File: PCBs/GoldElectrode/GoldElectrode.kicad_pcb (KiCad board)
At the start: 2 copper layers, 30 x 51 mm, 2 parts, among them J1 Finger, J2 Pad

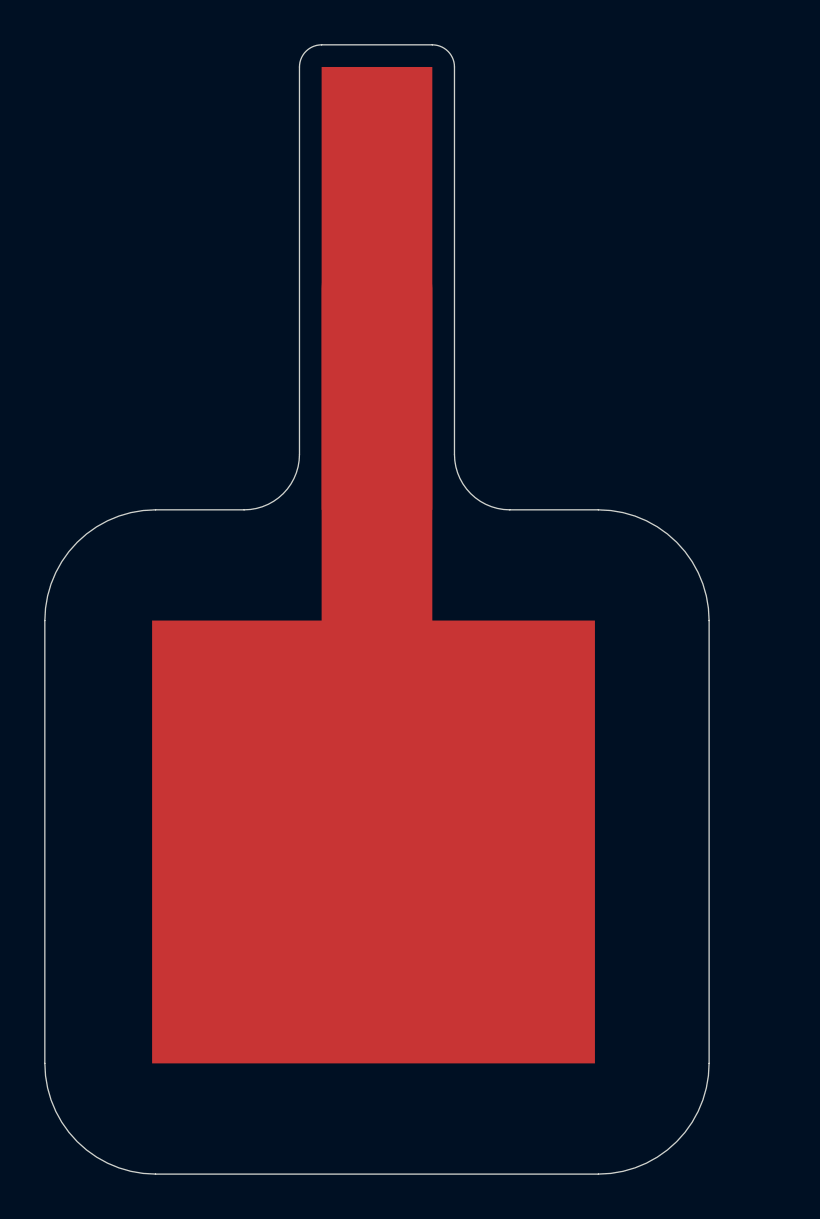
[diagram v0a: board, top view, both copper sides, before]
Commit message: kicad changes
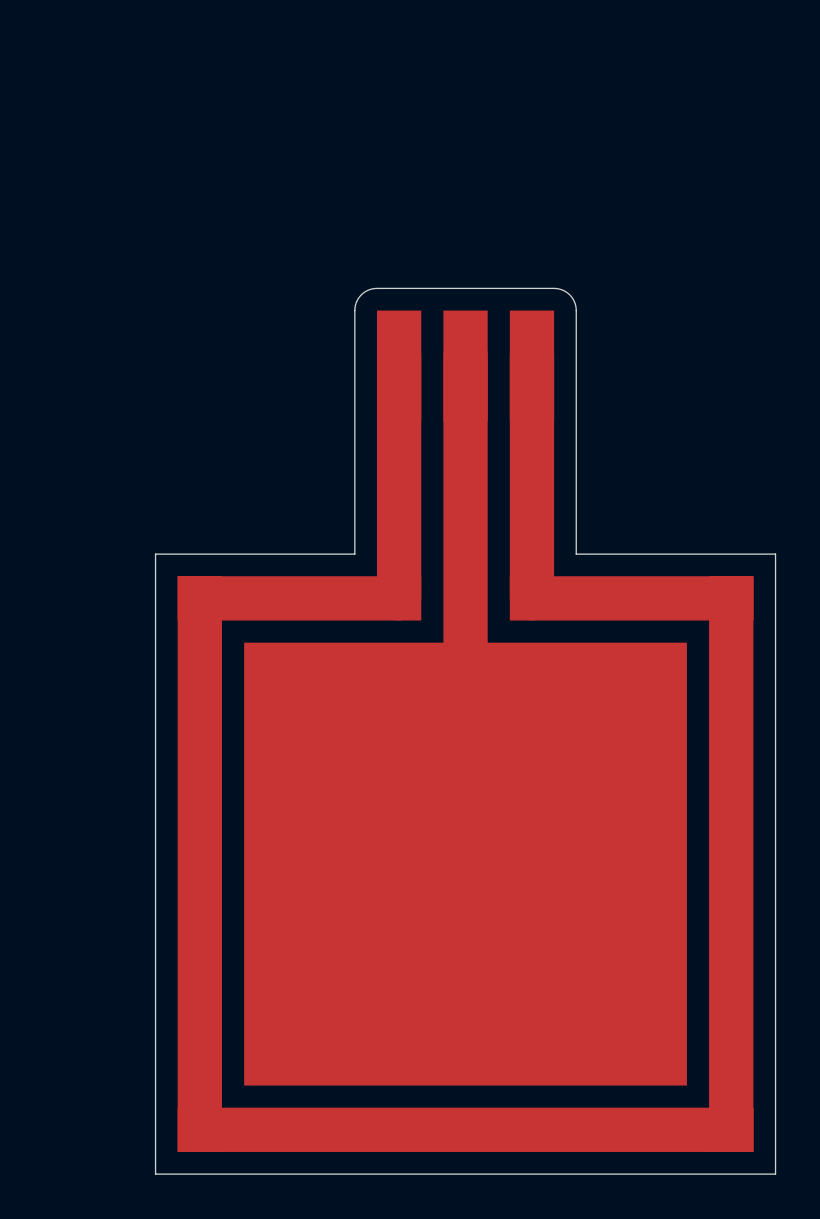
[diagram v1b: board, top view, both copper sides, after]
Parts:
- removed J1: Finger, 4022S:Finger_01
- removed J2: Pad, 4022S:Pad_20x20_mm
- added J3: Pad, 4022S:Gold_electrode_pad, F.Cu at (109.0, 76.0)
- added J4: Finger, 4022S:Gold_electrode_finger, F.Cu at (109.0, 53.5)
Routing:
- net Net-(J1-Pin_1): track 25.1 -> 0.00 mm
- net /Pad: track 0.00 -> 23.0 mm
- net /Fringe Shield: track 0.00 -> 22.0 mm
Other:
- board size 30 x 51 mm -> 28 x 40 mm
